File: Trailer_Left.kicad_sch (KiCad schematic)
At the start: 11 parts, among them Q20 IRLZ44N, SW4 SW_SPST, U5 LM339

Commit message: Add files via upload
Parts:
- R67: footprint Resistor_THT:R_Axial_Power_L25.0mm_W9.0mm_P27.94mm -> Resistor_THT:R_Axial_DIN0207_L6.3mm_D2.5mm_P10.16mm_Horizontal
- R68, R69: footprint TRIM_3296W1103LF:TRIM_3296W1103LF -> (none)
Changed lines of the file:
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@@
 			)
 		)
-		(property "Footprint" "Resistor_THT:R_Axial_Power_L25.0mm_W9.0mm_P27.94mm"
+		(property "Footprint" "Resistor_THT:R_Axial_DIN0207_L6.3mm_D2.5mm_P10.16mm_Horizontal"
 			(at 83.439 84.328 0)
 			(hide yes)
@@
 			)
 		)
-		(property "Footprint" "TRIM_3296W1103LF:TRIM_3296W1103LF"
+		(property "Footprint" ""
 			(at 95.25 66.04 0)
 			(hide yes)
@@
 			)
 		)
-		(property "Footprint" "TRIM_3296W1103LF:TRIM_3296W1103LF"
+		(property "Footprint" ""
 			(at 106.68 87.63 0)
 			(hide yes)

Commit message: Add files via upload
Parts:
- R67: footprint Resistor_THT:R_Axial_DIN0207_L6.3mm_D2.5mm_P10.16mm_Horizontal -> Resistor_THT:R_Axial_Power_L25.0mm_W9.0mm_P27.94mm
- R68, R69: footprint (none) -> TRIM_3296W1103LF:TRIM_3296W1103LF
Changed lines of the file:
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@@
 			)
 		)
-		(property "Footprint" "Resistor_THT:R_Axial_DIN0207_L6.3mm_D2.5mm_P10.16mm_Horizontal"
+		(property "Footprint" "Resistor_THT:R_Axial_Power_L25.0mm_W9.0mm_P27.94mm"
 			(at 83.439 84.328 0)
 			(hide yes)
@@
 			)
 		)
-		(property "Footprint" ""
+		(property "Footprint" "TRIM_3296W1103LF:TRIM_3296W1103LF"
 			(at 95.25 66.04 0)
 			(hide yes)
@@
 			)
 		)
-		(property "Footprint" ""
+		(property "Footprint" "TRIM_3296W1103LF:TRIM_3296W1103LF"
 			(at 106.68 87.63 0)
 			(hide yes)

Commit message: Add files via upload
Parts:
- U5: footprint (none) -> Package_DIP:DIP-14_W7.62mm_Socket
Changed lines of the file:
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@@
 			)
 		)
-		(property "Footprint" ""
+		(property "Footprint" "Package_DIP:DIP-14_W7.62mm_Socket"
 			(at 135.89 43.18 0)
 			(hide yes)
@@
 			)
 		)
-		(property "Footprint" ""
+		(property "Footprint" "Package_DIP:DIP-14_W7.62mm_Socket"
 			(at 135.89 62.23 0)
 			(hide yes)
@@
 			)
 		)
-		(property "Footprint" ""
+		(property "Footprint" "Package_DIP:DIP-14_W7.62mm_Socket"
 			(at 135.89 83.82 0)
 			(hide yes)
@@
 			)
 		)
-		(property "Footprint" ""
+		(property "Footprint" "Package_DIP:DIP-14_W7.62mm_Socket"
 			(at 137.16 101.6 0)
 			(hide yes)
@@
 			)
 		)
-		(property "Footprint" ""
+		(property "Footprint" "Package_DIP:DIP-14_W7.62mm_Socket"
 			(at 124.46 121.92 0)
 			(hide yes)

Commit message: Add files via upload
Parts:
- U5: footprint Package_DIP:DIP-14_W7.62mm_Socket -> (none)
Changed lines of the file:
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@@
 			)
 		)
-		(property "Footprint" "Package_DIP:DIP-14_W7.62mm_Socket"
+		(property "Footprint" ""
 			(at 135.89 43.18 0)
 			(hide yes)
@@
 			)
 		)
-		(property "Footprint" "Package_DIP:DIP-14_W7.62mm_Socket"
+		(property "Footprint" ""
 			(at 135.89 62.23 0)
 			(hide yes)
@@
 			)
 		)
-		(property "Footprint" "Package_DIP:DIP-14_W7.62mm_Socket"
+		(property "Footprint" ""
 			(at 135.89 83.82 0)
 			(hide yes)
@@
 			)
 		)
-		(property "Footprint" "Package_DIP:DIP-14_W7.62mm_Socket"
+		(property "Footprint" ""
 			(at 137.16 101.6 0)
 			(hide yes)
@@
 			)
 		)
-		(property "Footprint" "Package_DIP:DIP-14_W7.62mm_Socket"
+		(property "Footprint" ""
 			(at 124.46 121.92 0)
 			(hide yes)

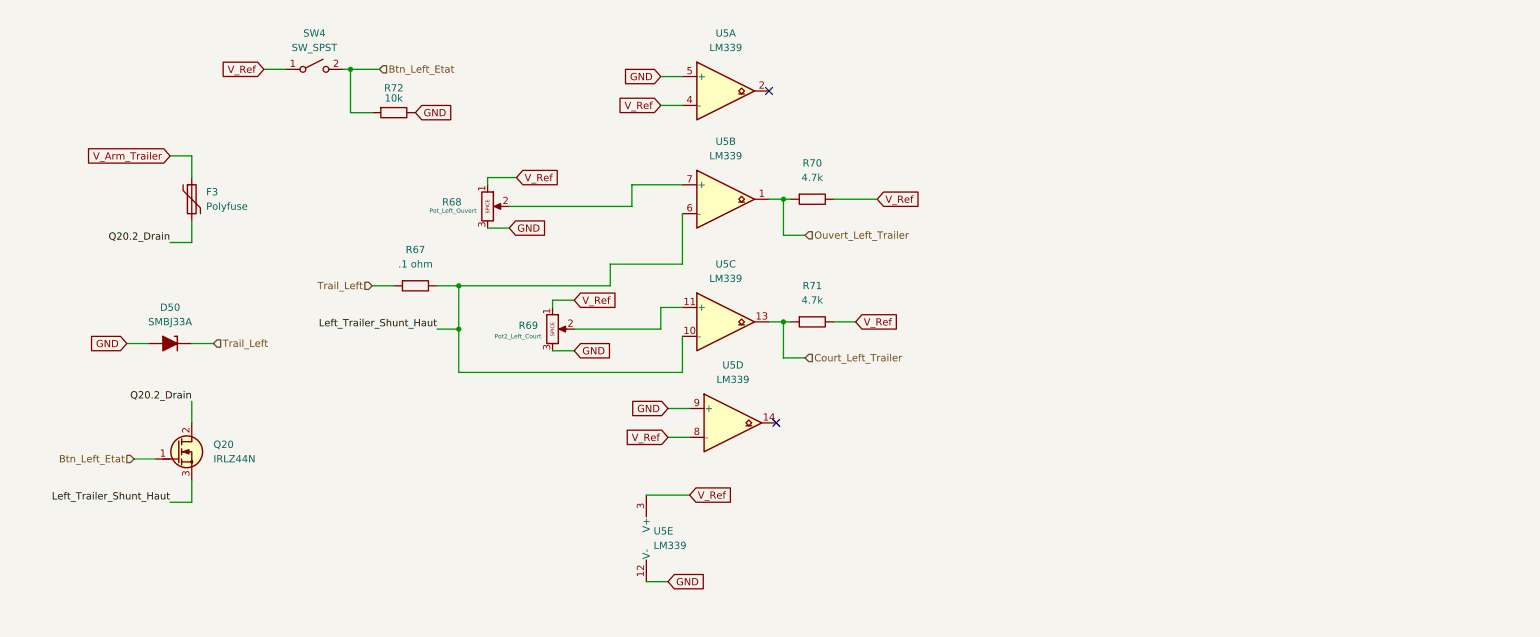
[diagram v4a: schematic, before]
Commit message: Add files via upload
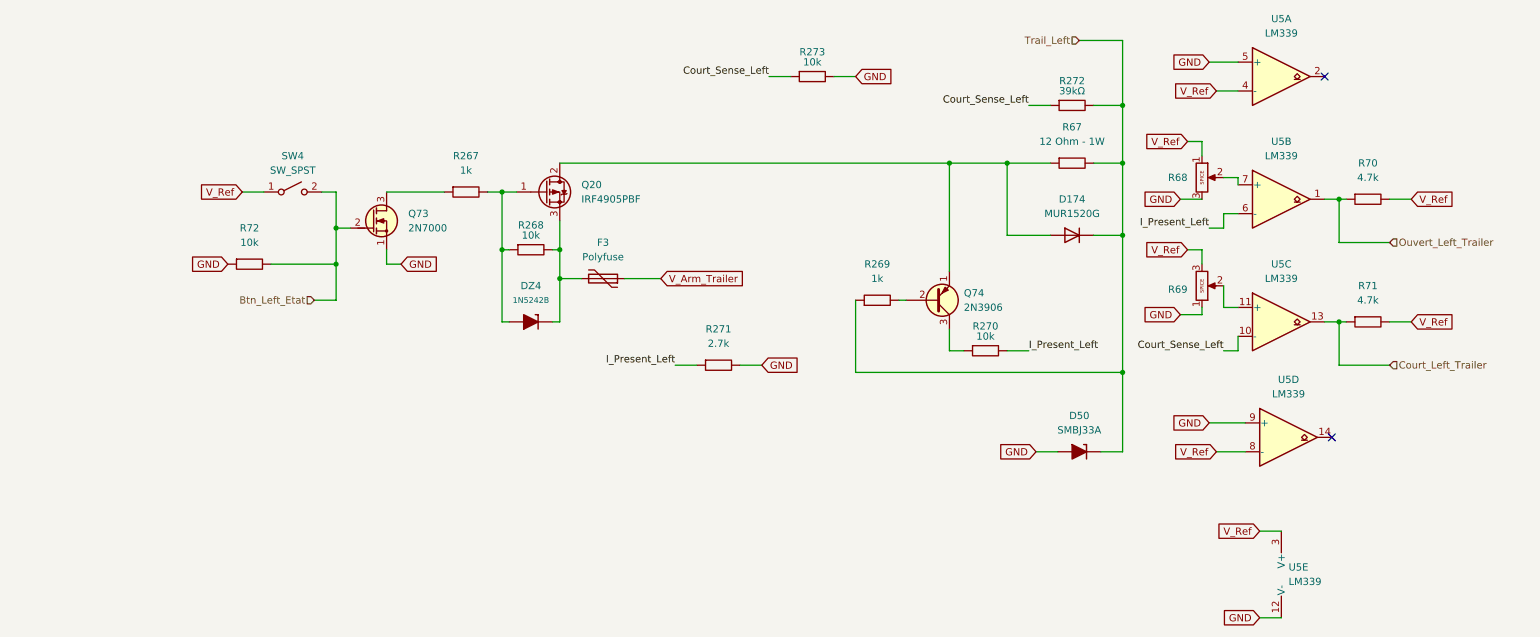
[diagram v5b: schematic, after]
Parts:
- removed Q20: IRLZ44N, PCM_Package_TO_SOT_THT_AKL:TO-220-3_Vertical_GDS, symbol PCM_Transistor_MOSFET_AKL:IRLZ44N
- removed R67: .1 ohm, Resistor_THT:R_Axial_Power_L25.0mm_W9.0mm_P27.94mm, symbol PCM_SL_Resistors:4.7k
- removed R72: 10k, Resistor_THT:R_Axial_DIN0207_L6.3mm_D2.5mm_P10.16mm_Horizontal, symbol PCM_SL_Resistors:10k
- added D174: MUR1520G, Package_TO_SOT_THT:TO-220-2_Vertical, symbol Device:D
- added DZ4: 1N5242B, PCM_Diode_THT_AKL:D_DO-35_SOD27_P7.62mm_Horizontal_Zener, symbol PCM_Diode_Zener_AKL:1N5242B
- added Q20: IRF4905PBF, Package_TO_SOT_THT:TO-220-3_Vertical, symbol Transistor_FET:IRF4905
- added Q73: 2N7000, PCM_Package_TO_SOT_THT_AKL:TO-92_Inline_Wide_SGD, symbol PCM_Transistor_MOSFET_AKL:2N7000
- added Q74: 2N3906, PCM_Package_TO_SOT_THT_AKL:TO-92_Inline_Wide_EBC, symbol PCM_Transistor_BJT_AKL:2N3906
- added R267, R269: 1k, Resistor_THT:R_Axial_DIN0207_L6.3mm_D2.5mm_P10.16mm_Horizontal, symbol PCM_SL_Resistors:1k
- added R268, R270, R273: 10k, Resistor_THT:R_Axial_DIN0207_L6.3mm_D2.5mm_P10.16mm_Horizontal, symbol PCM_SL_Resistors:10k
- added R271: 2.7k, Resistor_THT:R_Axial_DIN0207_L6.3mm_D2.5mm_P10.16mm_Horizontal, symbol PCM_SL_Resistors:2.7k
- added R272: 39kΩ, Resistor_THT:R_Axial_DIN0207_L6.3mm_D2.5mm_P10.16mm_Horizontal, symbol PCM_SL_Resistors:10k
- added R67: 12 Ohm - 1W, Resistor_THT:R_Axial_DIN0414_L11.9mm_D4.5mm_P15.24mm_Horizontal, symbol PCM_SL_Devices:Resistor_5W
- added R72: 10k, Resistor_THT:R_Axial_DIN0207_L6.3mm_D2.5mm_P10.16mm_Horizontal, symbol PCM_SL_Resistors:4.7k
- R68: Etiquette Pot_Left_Ouvert -> (none)
- R69: Etiquette Pot2_Left_Court -> (none)
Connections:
- net Btn_Left_Etat: now also Q73.2 (G), R72.2
- net GND: now also R69.1, Q73.1 (S), R271.2, R273.2, R72.1; no longer R69.3
- net Trail_Left: now also D174.1 (K), R269.1, R272.2, R67.2
- net V_Ref: now also R69.3; no longer R69.1
- net Left_Trailer_Shunt_Haut renamed Court_Sense_Left
- net Court_Sense_Left: now also R272.1, R273.1; no longer U5.6 (-)
- net Q20.2_Drain: no longer names the net of F3.2
- net Q20.2_Drain: now also DZ4.1 (K), Q20.3 (S), R268.2
- new net: DZ4.2 (A), Q20.1 (G), R267.2, R268.1
- new net: D174.2 (A), Q20.2 (D), Q74.1 (E), R67.1
- new net: Q73.3 (D), R267.1
- new net: Q74.2 (B), R269.2
- new net: Q74.3 (C), R270.1
- new net I_Present_Left: R270.2, R271.1, U5.6 (-)
